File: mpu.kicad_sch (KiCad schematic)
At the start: 27 parts, among them J12 Conn_01x06, U2 STM32U585CIUxQ, Y1 ECS-160-8-36B2-CKM-TR, Y2 CM7V-T1A-32.768KHZ

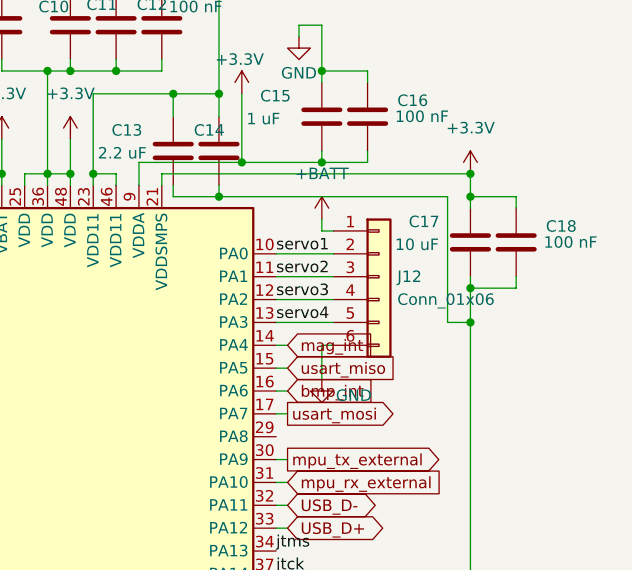
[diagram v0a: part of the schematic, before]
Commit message: worked mainly on pcb
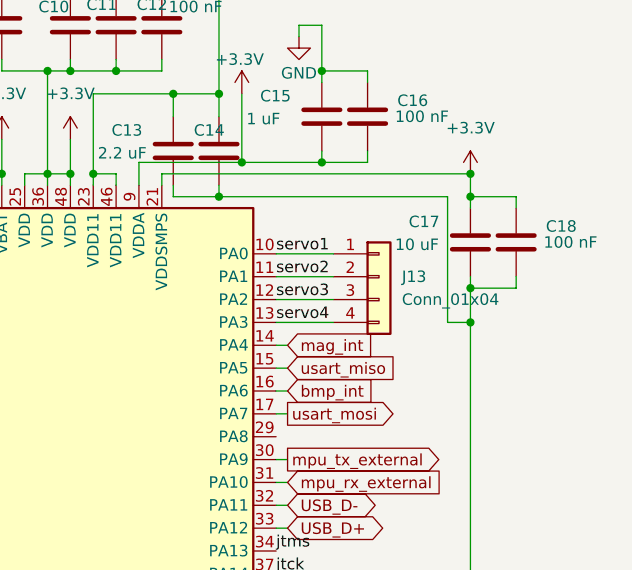
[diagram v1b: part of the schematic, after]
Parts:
- removed J12: Conn_01x06, Connector_PinHeader_2.54mm:PinHeader_1x06_P2.54mm_Vertical, symbol Connector_Generic:Conn_01x06
- added J13: Conn_01x04, Connector_PinHeader_2.54mm:PinHeader_1x04_P2.54mm_Vertical, symbol Connector_Generic:Conn_01x04
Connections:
- net servo1: now also J13.1 (Pin_1)
- net servo2: now also J13.2 (Pin_2)
- net servo3: now also J13.3 (Pin_3)
- net servo4: now also J13.4 (Pin_4)
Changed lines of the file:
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@@
 	(wire
 		(pts
-			(xy 163.83 76.2) (xy 163.83 77.47)
-		)
-		(stroke
-			(width 0)
-			(type default)
-		)
-	)
-	(wire
-		(pts
 			(xy 111.76 125.73) (xy 113.03 125.73)
 		)
@@
 	(wire
 		(pts
-			(xy 158.75 90.17) (xy 160.02 90.17)
-		)
-		(stroke
-			(width 0)
-			(type default)
-		)
-	)
-	(wire
-		(pts
 			(xy 109.22 80.01) (xy 113.03 80.01)
 		)
@@
 	(wire
 		(pts
-			(xy 163.83 93.98) (xy 163.83 90.17)
-		)
-		(stroke
-			(width 0)
-			(type default)
-		)
-	)
-	(wire
-		(pts
 			(xy 138.43 72.39) (xy 138.43 71.12)
 		)
@@
 	(wire
 		(pts
-			(xy 163.83 90.17) (xy 165.1 90.17)
-		)
-		(stroke
-			(width 0)
-			(type default)
-		)
-	)
-	(wire
-		(pts
 			(xy 58.42 87.63) (xy 58.42 92.71)
 		)
@@
 	(wire
 		(pts
-			(xy 140.97 49.53) (xy 140.97 50.8)
+			(xy 158.75 90.17) (xy 160.02 90.17)
 		)
 		(stroke
@@
 	(wire
 		(pts
-			(xy 138.43 71.12) (xy 138.43 62.23)
+			(xy 140.97 49.53) (xy 140.97 50.8)
 		)
 		(stroke
@@
 	(wire
 		(pts
-			(xy 133.35 43.18) (xy 135.89 43.18)
+			(xy 138.43 71.12) (xy 138.43 62.23)
 		)
 		(stroke
@@
 	(wire
 		(pts
-			(xy 67.31 93.98) (xy 67.31 95.25)
+			(xy 133.35 43.18) (xy 135.89 43.18)
 		)
 		(stroke
@@
 	(wire
 		(pts
-			(xy 128.27 71.12) (xy 128.27 72.39)
+			(xy 67.31 93.98) (xy 67.31 95.25)
 		)
 		(stroke
@@
 	(wire
 		(pts
-			(xy 113.03 100.33) (xy 111.76 100.33)
+			(xy 128.27 71.12) (xy 128.27 72.39)
 		)
 		(stroke
@@
 	(wire
 		(pts
-			(xy 111.76 110.49) (xy 113.03 110.49)
+			(xy 113.03 100.33) (xy 111.76 100.33)
 		)
 		(stroke
@@
 	(wire
 		(pts
-			(xy 163.83 77.47) (xy 165.1 77.47)
+			(xy 111.76 110.49) (xy 113.03 110.49)
 		)
 		(stroke
@@
 	)
 	(symbol
+		(lib_id "Connector_Generic:Conn_01x04")
+		(at 170.18 82.55 0)
+		(unit 1)
+		(exclude_from_sim no)
+		(in_bom yes)
+		(on_board yes)
+		(dnp no)
+		(fields_autoplaced yes)
+		(property "Reference" "J13"
+			(at 172.72 82.5499 0)
+			(effects
+				(font
+					(size 1.27 1.27)
+				)
+				(justify left)
+			)
+		)
+		(property "Value" "Conn_01x04"
+			(at 172.72 85.0899 0)
+			(effects
+				(font
+					(size 1.27 1.27)
+				)
+				(justify left)
+			)
+		)
+		(property "Footprint" "Connector_PinHeader_2.54mm:PinHeader_1x04_P2.54mm_Vertical"
+			(at 170.18 82.55 0)
+			(effects
+				(font
+					(size 1.27 1.27)
+				)
+				(hide yes)
+			)
+		)
+		(property "Datasheet" "~"
+			(at 170.18 82.55 0)
+			(effects
+				(font
+					(size 1.27 1.27)
+				)
+				(hide yes)
+			)
+		)
+		(property "Description" "Generic connector, single row, 01x04, script generated (kicad-library-utils/schlib/autogen/connector/)"
+			(at 170.18 82.55 0)
+			(effects
+				(font
+					(size 1.27 1.27)
+				)
+				(hide yes)
+			)
+		)
+		(pin "4"
+		)
+		(pin "2"
+		)
+		(pin "1"
+		)
+		(pin "3"
+		)
+		(instances
+			(project ""
+				(path "/d0cafa98-cc2a-4ab3-8dbc-f937bedf434b/94fda4c7-40dd-4c5d-acdd-b2f66ff666c2"
+					(reference "J13")
+					(unit 1)
+				)
+			)
+		)
+	)
+	(symbol
 		(lib_id "Connector_Generic:Conn_01x02")
 		(at 102.87 74.93 90)
@@
 	)
 	(symbol
-		(lib_id "power:+BATT")
-		(at 163.83 76.2 0)
-		(unit 1)
-		(exclude_from_sim no)
-		(in_bom yes)
-		(on_board yes)
-		(dnp no)
-		(fields_autoplaced yes)
-		(property "Reference" "#PWR029"
-			(at 163.83 80.01 0)
-			(effects
-				(font
-					(size 1.27 1.27)
-				)
-				(hide yes)
-			)
-		)
-		(property "Value" "+BATT"
-			(at 163.83 71.12 0)
-			(effects
-				(font
-					(size 1.27 1.27)
-				)
-			)
-		)
-		(property "Footprint" ""
-			(at 163.83 76.2 0)
-			(effects
-				(font
-					(size 1.27 1.27)
-				)
-				(hide yes)
-			)
-		)
-		(property "Datasheet" ""
-			(at 163.83 76.2 0)
-			(effects
-				(font
-					(size 1.27 1.27)
-				)
-				(hide yes)
-			)
-		)
-		(property "Description" "Power symbol creates a global label with name \"+BATT\""
-			(at 163.83 76.2 0)
-			(effects
-				(font
-					(size 1.27 1.27)
-				)
-				(hide yes)
-			)
-		)
-		(pin "1"
-		)
-		(instances
-			(project ""
-				(path "/d0cafa98-cc2a-4ab3-8dbc-f937bedf434b/94fda4c7-40dd-4c5d-acdd-b2f66ff666c2"
-					(reference "#PWR029")
-					(unit 1)
-				)
-			)
-		)
-	)
-	(symbol
 		(lib_id "Connector_Generic:Conn_01x02")
 		(at 69.85 100.33 270)
@@
 	)
 	(symbol
-		(lib_id "power:GND")
-		(at 163.83 93.98 0)
-		(unit 1)
-		(exclude_from_sim no)
-		(in_bom yes)
-		(on_board yes)
-		(dnp no)
-		(property "Reference" "#PWR090"
-			(at 163.83 100.33 0)
-			(effects
-				(font
-					(size 1.27 1.27)
-				)
-				(hide yes)
-			)
-		)
-		(property "Value" "GND"
-			(at 167.386 95.758 0)
-			(effects
-				(font
-					(size 1.27 1.27)
-				)
-			)
-		)
-		(property "Footprint" ""
-			(at 163.83 93.98 0)
-			(effects
-				(font
-					(size 1.27 1.27)
-				)
-				(hide yes)
-			)
-		)
-		(property "Datasheet" ""
-			(at 163.83 93.98 0)
-			(effects
-				(font
-					(size 1.27 1.27)
-				)
-				(hide yes)
-			)
-		)
-		(property "Description" "Power symbol creates a global label with name \"GND\" , ground"
-			(at 163.83 93.98 0)
-			(effects
-				(font
-					(size 1.27 1.27)
-				)
-				(hide yes)
-			)
-		)
-		(pin "1"
-		)
-		(instances
-			(project ""
-				(path "/d0cafa98-cc2a-4ab3-8dbc-f937bedf434b/94fda4c7-40dd-4c5d-acdd-b2f66ff666c2"
-					(reference "#PWR090")
-					(unit 1)
-				)
-			)
-		)
-	)
-	(symbol
 		(lib_id "ECS-160-8-36B2-CKM-TR:ECS-160-8-36B2-CKM-TR")
 		(at 91.44 85.09 180)
@@
 					(unit 1)
 				)
-			)
-		)
-	)
-	(symbol
-		(lib_id "Connector_Generic:Conn_01x06")
-		(at 170.18 82.55 0)
-		(unit 1)
-		(exclude_from_sim no)
-		(in_bom yes)
-		(on_board yes)
-		(dnp no)
-		(property "Reference" "J12"
-			(at 172.212 82.55 0)
-			(effects
-				(font
-					(size 1.27 1.27)
-				)
-				(justify left)
-			)
-		)
-		(property "Value" "Conn_01x06"
-			(at 172.212 85.09 0)
-			(effects
-				(font
-					(size 1.27 1.27)
-				)
-				(justify left)
-			)
-		)
-		(property "Footprint" "Connector_PinHeader_2.54mm:PinHeader_1x06_P2.54mm_Vertical"
-			(at 170.18 82.55 0)
-			(effects
-				(font
-					(size 1.27 1.27)
-				)
-				(hide yes)
-			)
-		)
-		(property "Datasheet" "~"
-			(at 170.18 82.55 0)
-			(effects
-				(font
-					(size 1.27 1.27)
-				)
-				(hide yes)
-			)
-		)
-		(property "Description" "Generic connector, single row, 01x06, script generated (kicad-library-utils/schlib/autogen/connector/)"
-			(at 170.18 82.55 0)
-			(effects
-				(font
-					(size 1.27 1.27)
-				)
-				(hide yes)
-			)
-		)
-		(pin "1"
-		)
-		(pin "6"
-		)
-		(pin "2"
-		)
-		(pin "4"
-		)
-		(pin "5"
-		)
-		(pin "3"
-		)
-		(instances
-			(project ""
-				(path "/d0cafa98-cc2a-4ab3-8dbc-f937bedf434b/94fda4c7-40dd-4c5d-acdd-b2f66ff666c2"
-					(reference "J12")
-					(unit 1)
-				)
